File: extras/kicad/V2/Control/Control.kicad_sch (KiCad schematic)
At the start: 12 parts, among them J6 left, J7 right, U1 SparkFun-micromod

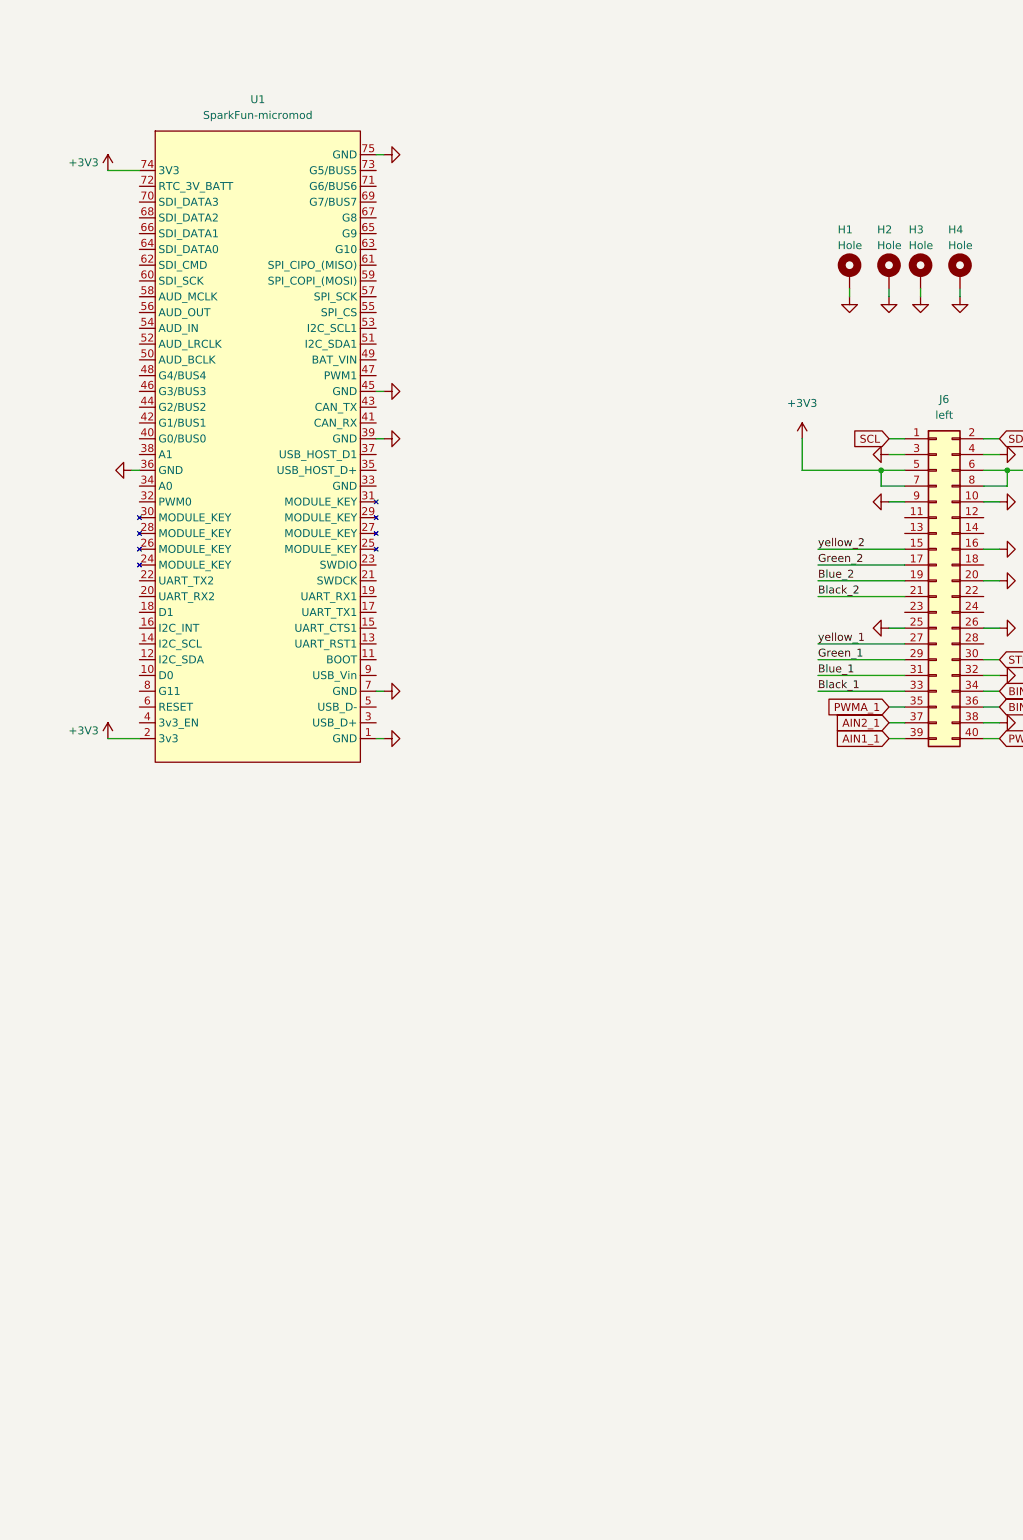
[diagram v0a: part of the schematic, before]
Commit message: t
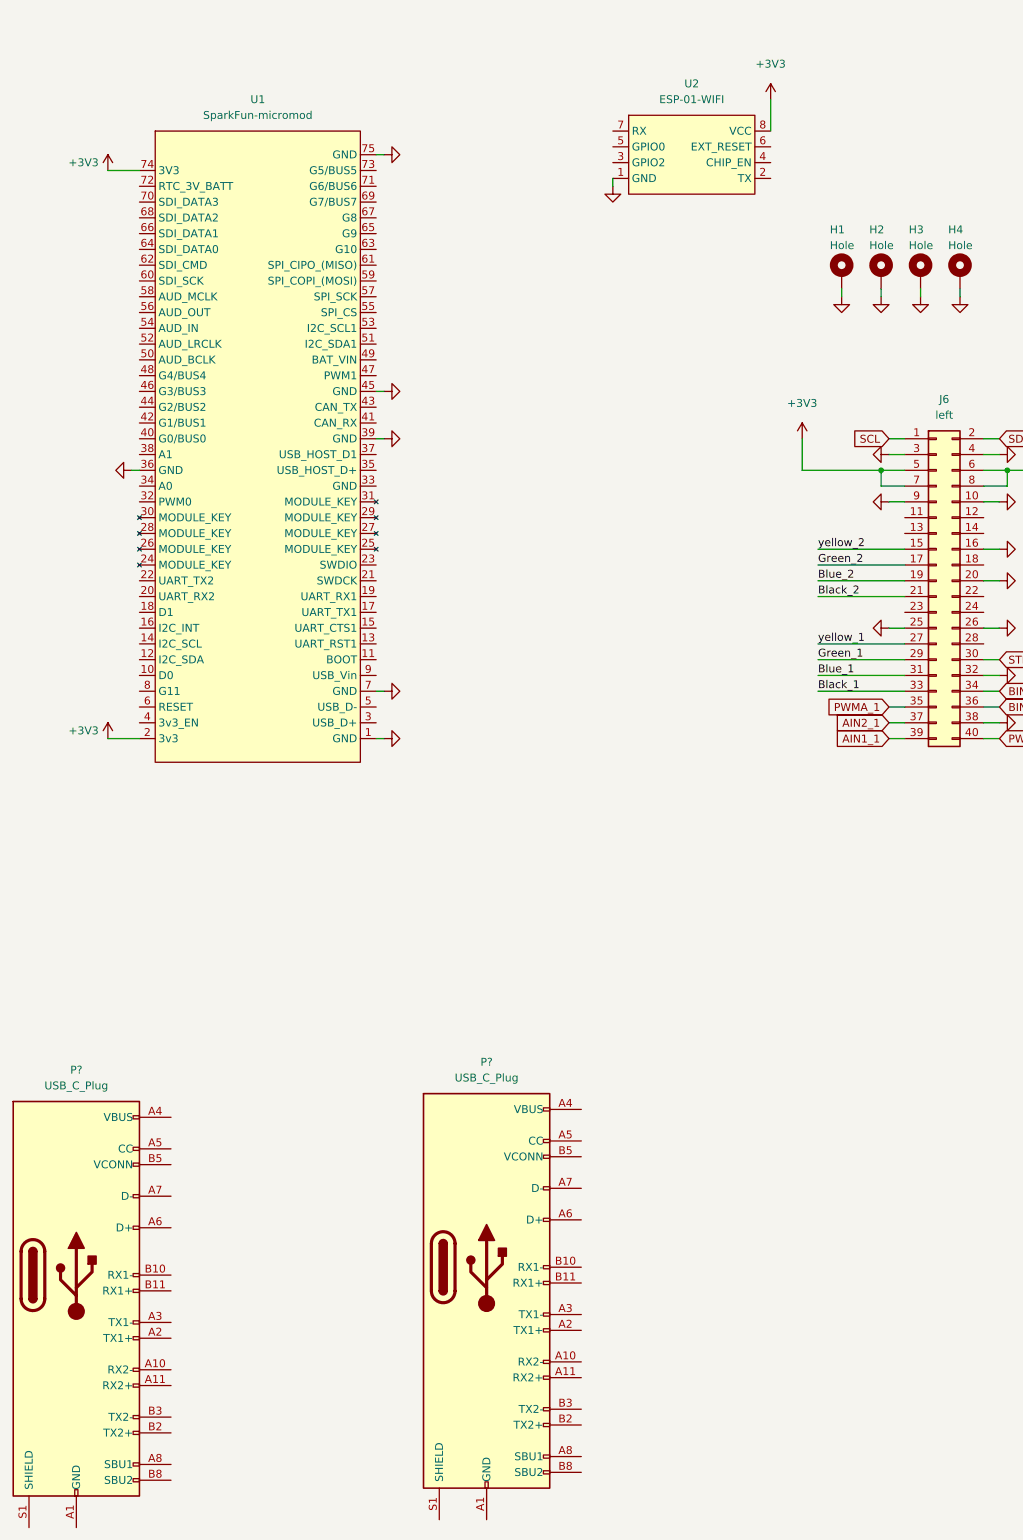
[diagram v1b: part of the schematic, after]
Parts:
- added P? (x2): USB_C_Plug, symbol Connector:USB_C_Plug
- added U2: ESP-01-WIFI, Connector_PinHeader_2.54mm:PinHeader_2x04_P2.54mm_Vertical, symbol My_custom_lib:ESP-01-WIFI
- U1: footprint (none) -> Z_mycustom_footprint_lib:SparkFun-micromod-footprint
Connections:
- net +3V3: now also U2.8 (VCC)
- net GND: now also U2.1 (GND)
- new net: P?.A1 (GND), P?.A12 (GND), P?.B1 (GND), P?.B12 (GND) (x2)
- new net: P?.A4 (VBUS), P?.A9 (VBUS), P?.B4 (VBUS), P?.B9 (VBUS) (x2)
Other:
- moved on the sheet: H1, H2

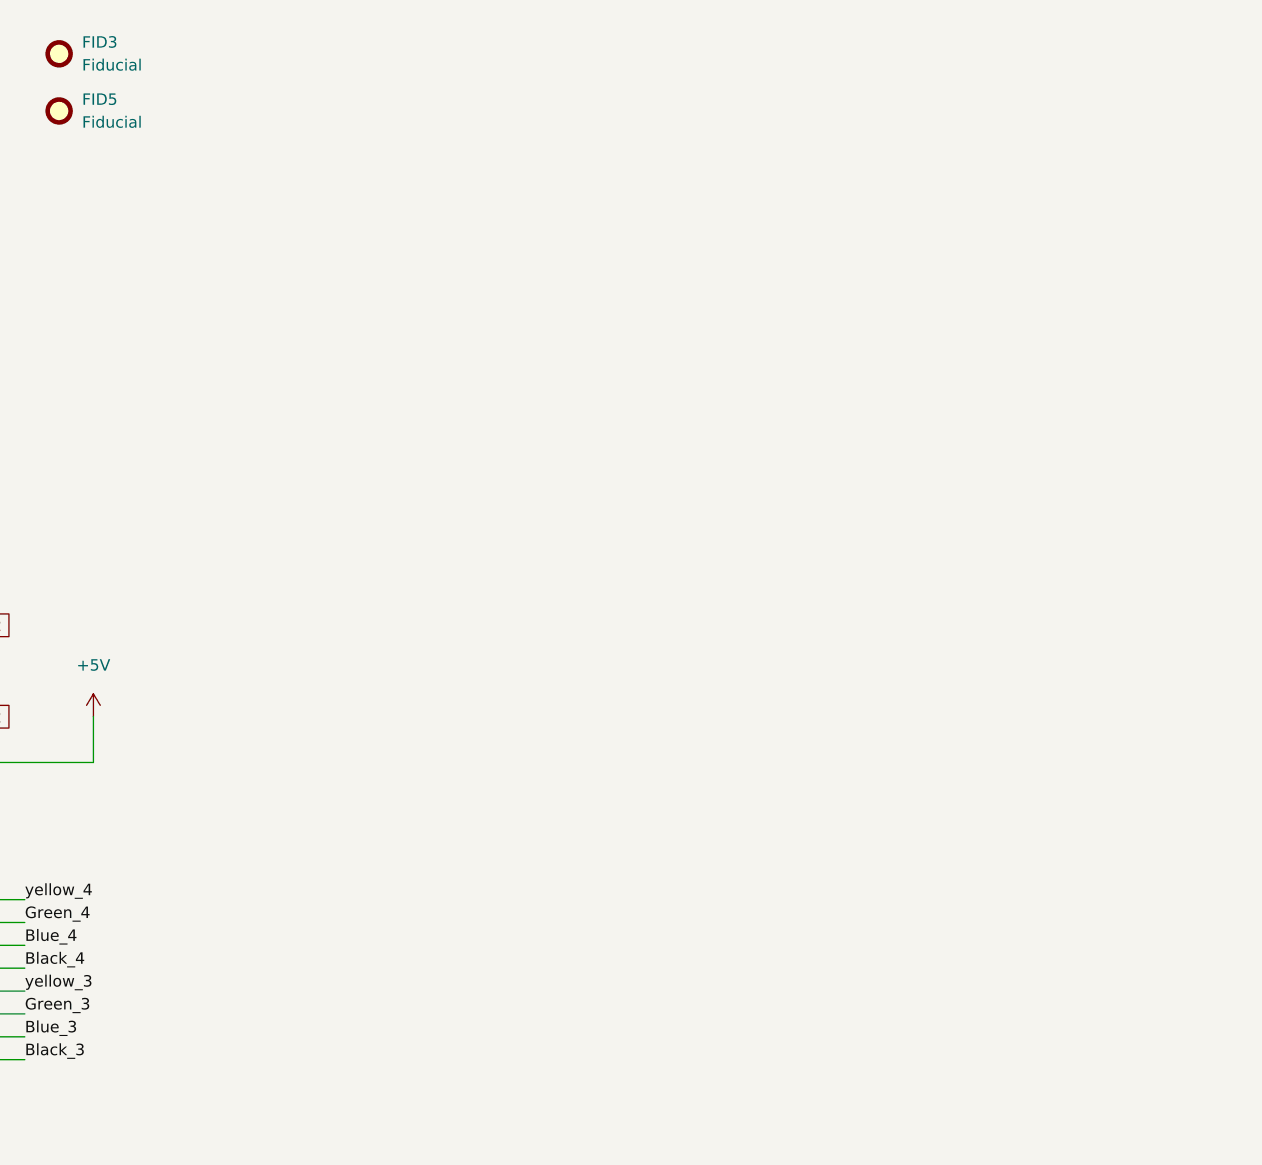
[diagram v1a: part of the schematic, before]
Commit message: g
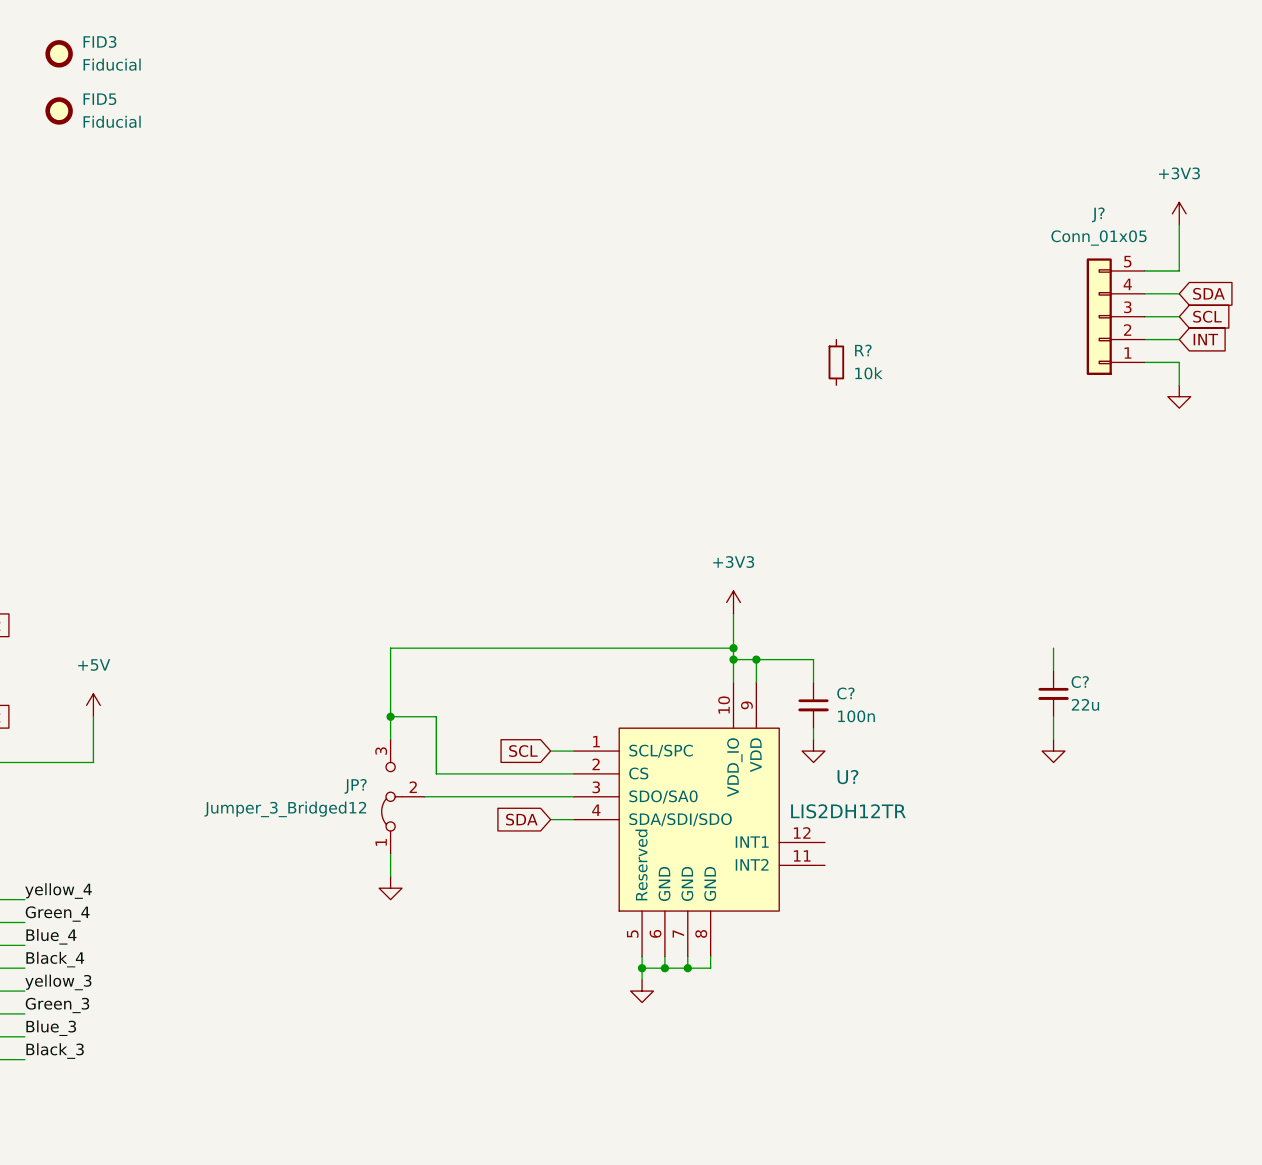
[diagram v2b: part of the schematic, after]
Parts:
- added C?: 22u, Capacitor_SMD:C_0805_2012Metric, symbol Device:C_Small
- added C?: 100n, Capacitor_SMD:C_0603_1608Metric, symbol Device:C_Small
- added J?: Conn_01x05, Connector_PinHeader_2.54mm:PinHeader_1x05_P2.54mm_Vertical, symbol Connector_Generic:Conn_01x05
- added JP?: Jumper_3_Bridged12, symbol Jumper:Jumper_3_Bridged12
- added R?: 10k, Resistor_SMD:R_0603_1608Metric, symbol Device:R_Small
- added U?: LIS2DH12TR, digikey-footprints:VFLGA-12_2x2mm, symbol dk_Motion-Sensors-Accelerometers:LIS2DH12TR
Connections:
- net +3V3: now also C?.1, J?.5 (Pin_5), JP?.3 (B), U?.10 (VDD_IO), U?.2 (CS), U?.9 (VDD)
- net GND: now also C?.2, C?.2, J?.1 (Pin_1), JP?.1 (A), U?.5 (Reserved), U?.6 (GND), U?.7 (GND), U?.8 (GND)
- net SCL: now also J?.3 (Pin_3), U?.1 (SCL/SPC)
- net SDA: now also J?.4 (Pin_4), U?.4 (SDA/SDI/SDO)
- new net: JP?.2 (C), U?.3 (SDO/SA0)
- new net INT: J?.2 (Pin_2)

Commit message: g
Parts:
- removed P? (x2): USB_C_Plug, symbol Connector:USB_C_Plug
- removed U?: LIS2DH12TR, digikey-footprints:VFLGA-12_2x2mm, symbol dk_Motion-Sensors-Accelerometers:LIS2DH12TR
- added C2: 100n, Capacitor_SMD:C_0603_1608Metric, symbol Device:C_Small
- added J1: Ultrasonic Ranging, Connector_PinHeader_2.54mm:PinHeader_1x04_P2.54mm_Vertical, symbol Connector_Generic:Conn_01x04
- added J? (x2): USB_C_Receptacle, symbol Connector:USB_C_Receptacle
- added R? (x4): 5k1, Resistor_SMD:R_0603_1608Metric, symbol Device:R_Small
- added TP1, TP2, TP3: TestPoint, TestPoint:TestPoint_Pad_1.5x1.5mm, symbol Connector:TestPoint
- added U3: LIS3DHTR, digikey-footprints:VFLGA-16_3x3mm, symbol dk_Motion-Sensors-Accelerometers:LIS3DHTR
- added U?: AI-64_headers, symbol My_custom_lib:AI-64_headers
- JP1: renamed from JP?; value Jumper_3_Bridged12 -> set; footprint (none) -> Jumper:SolderJumper-3_P1.3mm_Bridged12_Pad1.0x1.5mm; now left out of the parts list
- gave numbers to parts that had none: 4
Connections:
- net +3V3: now also C2.1, J1.4 (Pin_4), U3.1 (VDD_IO), U3.14 (VDD), U3.8 (CS)
- net GND: now also C2.2, J1.1 (Pin_1), J?.A1 (GND), J?.A1 (GND), J?.A12 (GND), J?.A12 (GND), J?.B1 (GND), J?.B1 (GND), J?.B12 (GND), J?.B12 (GND), J?.S1 (SHIELD), J?.S1 (SHIELD), R?.1, R?.1, R?.2, R?.2, U3.10 (Res), U3.12 (GND), U3.5 (GND)
- net SCL: now also U3.4 (SCL/SPC)
- net SDA: now also U3.6 (SDA/SDI/SDO)
- net at JP1.2 (C): now also U3.7 (SDO/SA0)
- new net: TP2.1, U3.15 (ADC2)
- new net: J?.A5 (CC1), R?.1 (x2)
- new net: J?.B5 (CC2), R?.2 (x2)
- new net: TP1.1, U3.13 (ADC3)
- new net: TP3.1, U3.16 (ADC1)
- new net: J?.A2 (TX1+), J?.A3 (TX1-) (x2)
- new net: J?.A4 (VBUS), J?.A9 (VBUS), J?.B4 (VBUS), J?.B9 (VBUS) (x2)
- new net: J?.B10 (RX1-), J?.B11 (RX1+) (x2)
- new net INT_1: U3.11 (INT1)
- new net INT_2: U3.9 (INT2)
- new net Sig: J1.2 (Pin_2)
- new net Trig: J1.3 (Pin_3)
- no-connect marks 0 -> 12
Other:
- note added: "I2C ardress: 001100X"
- moved on the sheet: C1, C3, JP1

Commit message: F
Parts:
- removed J? (x2): USB_C_Receptacle, symbol Connector:USB_C_Receptacle
- removed R? (x4): 5k1, Resistor_SMD:R_0603_1608Metric, symbol Device:R_Small
- removed U?: AI-64_headers, symbol My_custom_lib:AI-64_headers
- added C4: 100n, Capacitor_SMD:C_0603_1608Metric_Pad1.08x0.95mm_HandSolder, symbol Device:C_Small
- added C5: 15p, Capacitor_SMD:C_0603_1608Metric_Pad1.08x0.95mm_HandSolder, symbol Device:C_Small
- added J3: Output, Connector_USB:USB_C_Receptacle_HRO_TYPE-C-31-M-12, symbol Connector:USB_C_Receptacle
- added J4: Input, Connector_USB:USB_C_Receptacle_HRO_TYPE-C-31-M-12, symbol Connector:USB_C_Receptacle
- added JP2: set, Jumper:SolderJumper-3_P1.3mm_Bridged12_Pad1.0x1.5mm, symbol Jumper:Jumper_3_Bridged12
- added P8, P9: BeagleBone_Black_Header, Connector_PinHeader_2.54mm:PinHeader_2x23_P2.54mm_Vertical, symbol Connector_Generic:Conn_02x23_Odd_Even
- added R2: 2k7, Resistor_SMD:R_0603_1608Metric_Pad0.98x0.95mm_HandSolder, symbol Device:R_Small
- added R3, R4, R5, R6: 5k1, Resistor_SMD:R_0603_1608Metric_Pad0.98x0.95mm_HandSolder, symbol Device:R_Small
- added R7, R8: 1k, Resistor_SMD:R_0603_1608Metric_Pad0.98x0.95mm_HandSolder, symbol Device:R_Small
- added R9: 1Meg, Resistor_SMD:R_0603_1608Metric_Pad0.98x0.95mm_HandSolder, symbol Device:R_Small
- added U4: BNO085-breackout, Z_mycustom_footprint_lib:BNO085-breackout, symbol My_custom_lib:BNO085-breackout
- added U6: PCA9557PW, Package_SO:TSSOP-16_4.4x5mm_P0.65mm, symbol Interface_Expansion:PCA9557PW
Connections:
- net Black_1 is gone; now on net +3V3: J6.33 (Pin_33)
- net Black_2 is gone; now on net +3V3: J6.21 (Pin_21)
- net Black_3 is gone; now on net +3V3: J7.40 (Pin_40)
- net Black_4 is gone; now on net +3V3: J7.32 (Pin_32)
- net Blue_1 is gone; now on net +3V3: J6.31 (Pin_31)
- net Blue_2 is gone; now on net +3V3: J6.19 (Pin_19)
- net Blue_3 is gone; now on net +3V3: J7.38 (Pin_38)
- net Blue_4 is gone; now on net +3V3: J7.30 (Pin_30)
- net +3V3: now also C4.1, JP2.3 (B), P9.3 (Pin_3), P9.4 (Pin_4), R2.1, R7.1, R8.2, U4.1 (VIN), U6.16 (VDD)
- net +5V: now also P9.5 (Pin_5), P9.6 (Pin_6)
- net GND: now also C4.2, C5.2, J3.A1 (GND), J3.A12 (GND), J3.B1 (GND), J3.B12 (GND), J4.A1 (GND), J4.A12 (GND), J4.B1 (GND), J4.B12 (GND), JP2.1 (A), P8.1 (Pin_1), P8.2 (Pin_2), P8.45 (Pin_45), P9.1 (Pin_1), P9.2 (Pin_2), P9.34 (Pin_34), P9.43 (Pin_43), P9.44 (Pin_44), P9.45 (Pin_45), P9.46 (Pin_46), R3.2, R4.2, R5.2, R6.2, R9.1, U4.3 (GND), U6.5 (A2), U6.8 (VSS)
- net Green_1: now also U6.7 (IO1)
- net Green_2: now also U6.10 (IO3)
- net Green_3: now also U6.12 (IO5)
- net Green_4: now also U6.14 (IO7)
- net SCL: now also U4.4 (SCL), U6.1 (SCL)
- net SDA: now also U4.5 (SDA), U6.2 (SDA)
- net yellow_1: now also U6.6 (IO0)
- net yellow_2: now also U6.9 (IO2)
- net yellow_3: now also U6.11 (IO4)
- net yellow_4: now also U6.13 (IO6)
- new net: C5.1, J3.S1 (SHIELD), R9.2
- new net: JP2.2 (C), U4.8 (DI)
- new net: R8.1, U6.4 (A1)
- new net: R2.2, U6.15 (~{RESET})
- new net: R7.2, U6.3 (A0)
- new net +1V8: P9.32 (Pin_32)
- new net AIN0: P9.39 (Pin_39)
- new net AIN1: P9.40 (Pin_40)
- new net AIN2: P9.37 (Pin_37)
- new net AIN3: P9.38 (Pin_38)
- new net AIN4: P9.33 (Pin_33)
- new net AIN5: P9.36 (Pin_36)
- new net AIN6: P9.35 (Pin_35)
- new net D+: J3.A6 (D+), J3.B6 (D+)
- new net D-: J3.A7 (D-), J3.B7 (D-)
- new net D2+: J4.A6 (D+), J4.B6 (D+)
- new net D2-: J4.A7 (D-), J4.B7 (D-)
- new net GPIO[117]: P9.25 (Pin_25)
- new net GPIO[122]: P9.30 (Pin_30)
- new net GPIO[125]: P9.27 (Pin_27)
- new net GPIO[14]: P9.26 (Pin_26)
- new net GPIO[15]: P9.24 (Pin_24)
- new net GPIO[20]: P9.41 (Pin_41)
- new net GPIO[22]: P8.19 (Pin_19)
- new net GPIO[23]: P8.13 (Pin_13)
- new net GPIO[26]: P8.14 (Pin_14)
- new net GPIO[27]: P8.17 (Pin_17)
- new net GPIO[2]: P9.22 (Pin_22)
- new net GPIO[30]: P9.11 (Pin_11)
- new net GPIO[31]: P9.13 (Pin_13)
- new net GPIO[3]: P9.21 (Pin_21)
- new net GPIO[40]: P9.14 (Pin_14)
- new net GPIO[44]: P8.12 (Pin_12)
- new net GPIO[45]: P8.11 (Pin_11)
- new net GPIO[46]: P8.16 (Pin_16)
- new net GPIO[47]: P8.15 (Pin_15)
- new net GPIO[48]: P9.15 (Pin_15)
- new net GPIO[49]: P9.23 (Pin_23)
- new net GPIO[4]: P9.17 (Pin_17)
- new net GPIO[51]: P9.16 (Pin_16)
- new net GPIO[5]: P9.18 (Pin_18)
- new net GPIO[60]: P9.12 (Pin_12)
- new net GPIO[61]: P8.28 (Pin_28)
- new net GPIO[65]: P8.18 (Pin_18)
- new net GPIO[66]: P8.7 (Pin_7)
- new net GPIO[67]: P8.8 (Pin_8)
- new net GPIO[68]: P8.10 (Pin_10)
- new net GPIO[69]: P8.9 (Pin_9)
- new net GPIO[7]: P9.42 (Pin_42)
- new net I2C2.SCL: P9.19 (Pin_19)
- new net I2C2.SDA: P9.20 (Pin_20)
- new net LCD.AC_BIAS_E: P8.30 (Pin_30)
- new net LCD.DATA[0]: P8.43 (Pin_43)
- new net LCD.DATA[10]: P8.36 (Pin_36)
- new net LCD.DATA[11]: P8.34 (Pin_34)
- new net LCD.DATA[13]: P8.33 (Pin_33)
- new net LCD.DATA[14]: P8.31 (Pin_31)
- new net LCD.DATA[15]: P8.32 (Pin_32)
- new net LCD.DATA[1]: P8.46 (Pin_46)
- new net LCD.DATA[2]: P8.41 (Pin_41)
- new net LCD.DATA[3]: P8.44 (Pin_44)
- new net LCD.DATA[4]: P8.39 (Pin_39)
- new net LCD.DATA[5]: P8.42 (Pin_42)
- new net LCD.DATA[6]: P8.37 (Pin_37)
- new net LCD.DATA[7]: P8.40 (Pin_40)
- new net LCD.DATA[8]: P8.35 (Pin_35)
- new net LCD.DATA[9]: P8.38 (Pin_38)
- new net LCD.HSYNC: P8.29 (Pin_29)
- new net LCD.PCLK: P8.26 (Pin_26)
- new net LCD.VSYNC: P8.27 (Pin_27)
- new net MMC1.CLK: P8.21 (Pin_21)
- new net MMC1.CMD: P8.20 (Pin_20)
- new net MMC1.DAT[0]: P8.25 (Pin_25)
- new net MMC1.DAT[1]: P8.24 (Pin_24)
- new net MMC1.DAT[2]: P8.5 (Pin_5)
- new net MMC1.DAT[3]: P8.6 (Pin_6)
- new net MMC1.DAT[4]: P8.23 (Pin_23)
- new net MMC1.DAT[5]: P8.22 (Pin_22)
- new net MMC1.DAT[6]: P8.3 (Pin_3)
- new net MMC1.DAT[7]: P8.4 (Pin_4)
- new net PWR_BUT: P9.9 (Pin_9)
- new net SPI1.CS0: P9.28 (Pin_28)
- new net SPI1.D0: P9.29 (Pin_29)
- new net SPI1.SCLK: P9.31 (Pin_31)
- new net VBUS: J3.A4 (VBUS), J3.A9 (VBUS), J3.B4 (VBUS), J3.B9 (VBUS), J4.A4 (VBUS), J4.A9 (VBUS), J4.B4 (VBUS), J4.B9 (VBUS), P9.7 (Pin_7), P9.8 (Pin_8)
- new net cc1: J3.A5 (CC1), J4.A5 (CC1), R3.1, R4.1
- new net cc2: J3.B5 (CC2), J4.B5 (CC2), R5.1, R6.1
- new net ~{SYS_RESET}: P9.10 (Pin_10)
- no-connect marks 12 -> 28
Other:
- note added: "0011[A2][A1][A0]"
- note added: "100101X"
- moved on the sheet: C3
